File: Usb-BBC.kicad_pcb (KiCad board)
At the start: 2 copper layers, 34.3 x 22.9 mm, 24 parts, among them P1 USB_OTG, P2 BAT-Connector, P3 BAT-THT, P4 OUT-5V, SW1 SW_SPDT, U2 TP4056, U3 FS312F-G, U4 FS8205, U5 MT3608

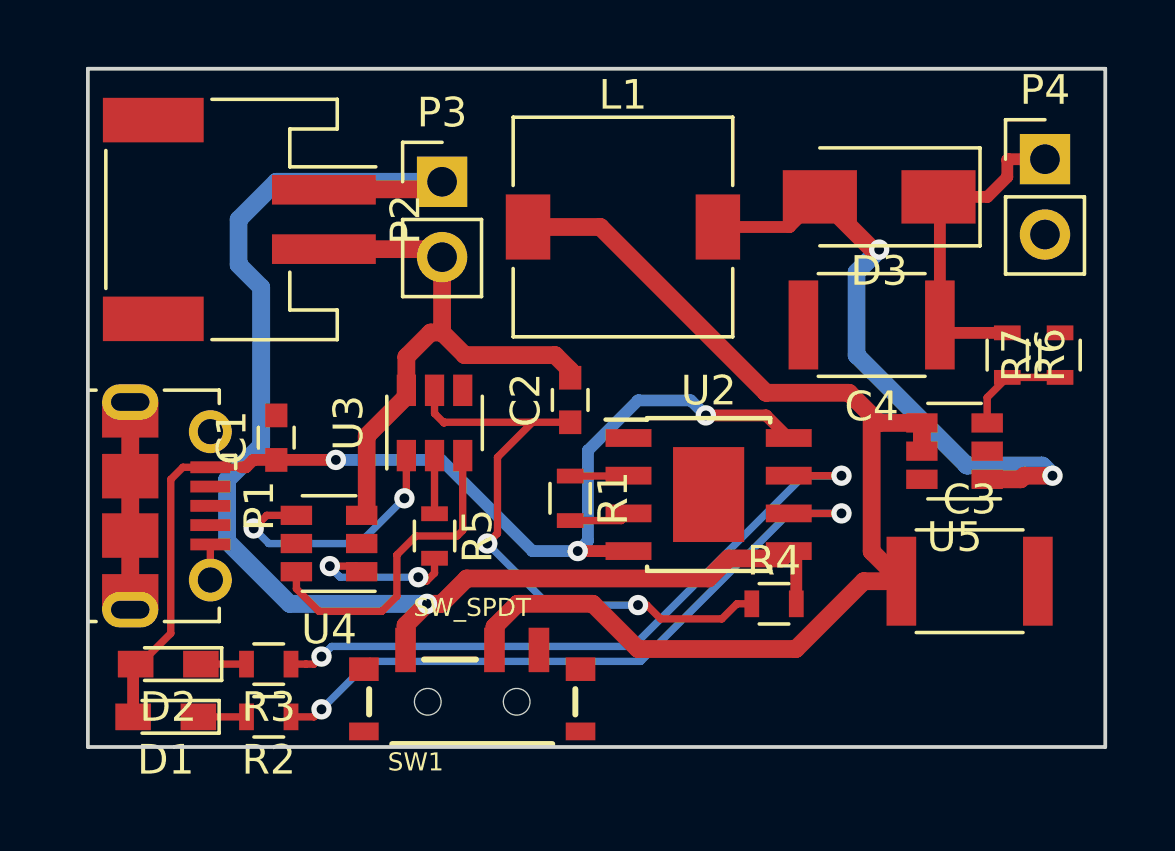
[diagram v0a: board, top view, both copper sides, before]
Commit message: Mandada a fabrica
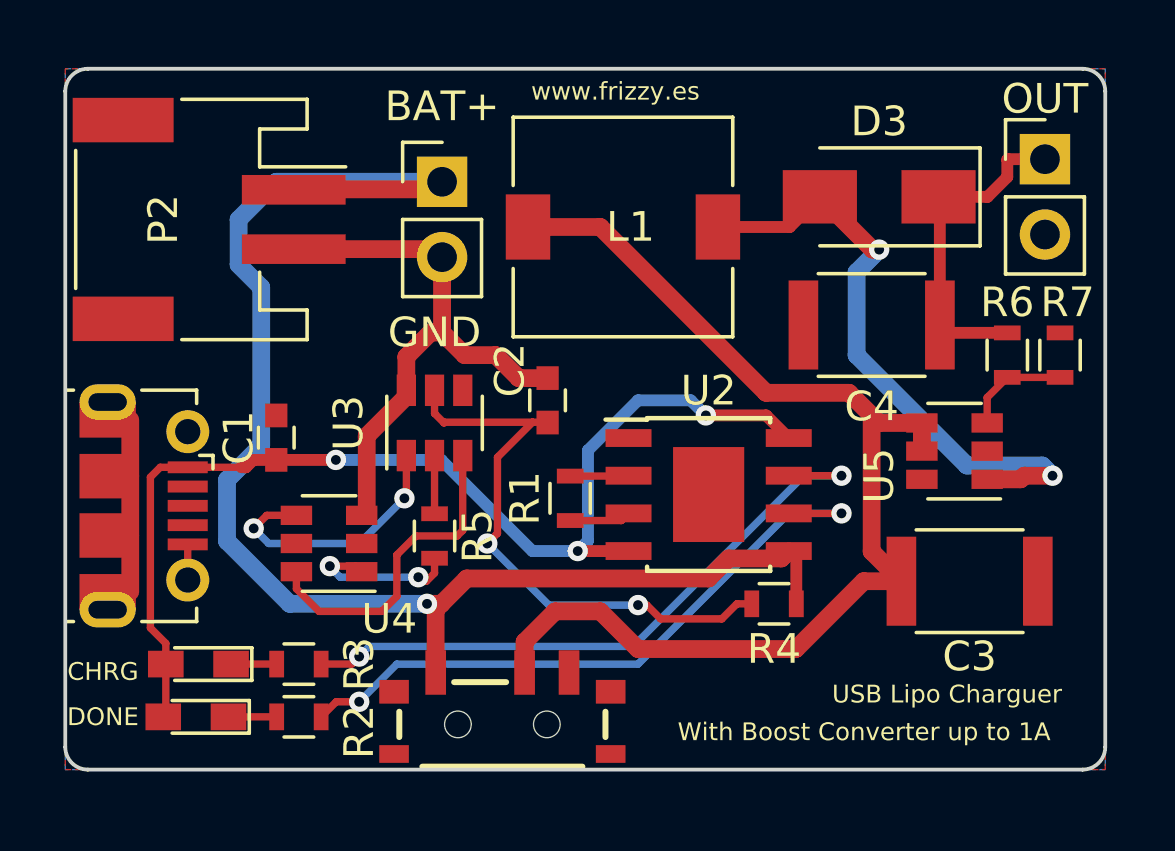
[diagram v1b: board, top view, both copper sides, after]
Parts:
- added G***: LOGO, logos_frizzy:glance, B.Cu at (149.1, 90.4)
- moved SW1 1.27 mm to (132.3, 92.5)
- moved D1 1.02 mm to (122.0, 92.2)
- moved D2 1.02 mm to (122.1, 90.4)
- moved P2 1.02 mm to (122.4, 75.4)
- moved R2 1.02 mm to (125.5, 92.2)
- moved R3 1.02 mm to (125.5, 90.4)
- moved C2 0.76 mm to (133.9, 81.5)
- moved P1 0.76 mm to (119.4, 85.1)
- renumbered P4 to OUT
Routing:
- net Net-(C3-Pad1): track 39.8 -> 38.6 mm
- net Net-(R3-Pad1): track 23.0 -> 21.9 mm
- net Net-(R2-Pad1): track 23.2 -> 22.2 mm
- net BAT-: track 18.9 -> 18.0 mm
- net Net-(C2-Pad1): track 20.4 -> 19.6 mm
- net BAT+: track 47.4 -> 47.9 mm
- added copper zone on B.Cu, net GND
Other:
- board size 34.3 x 22.9 mm -> 35.1 x 23.6 mm
- board text added: "+5V"
- board text added: "BAT+"
- board text added: "CHRG"
- board text added: "DONE"
- board text added: "GND"
- board text added: "OFF"
- board text added: "ON"
- board text added: "USB Lipo Charguer"
- board text added: "With Boost Converter up to 1A"
- board text added: "www.frizzy.es"
